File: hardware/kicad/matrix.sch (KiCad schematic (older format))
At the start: 14 parts

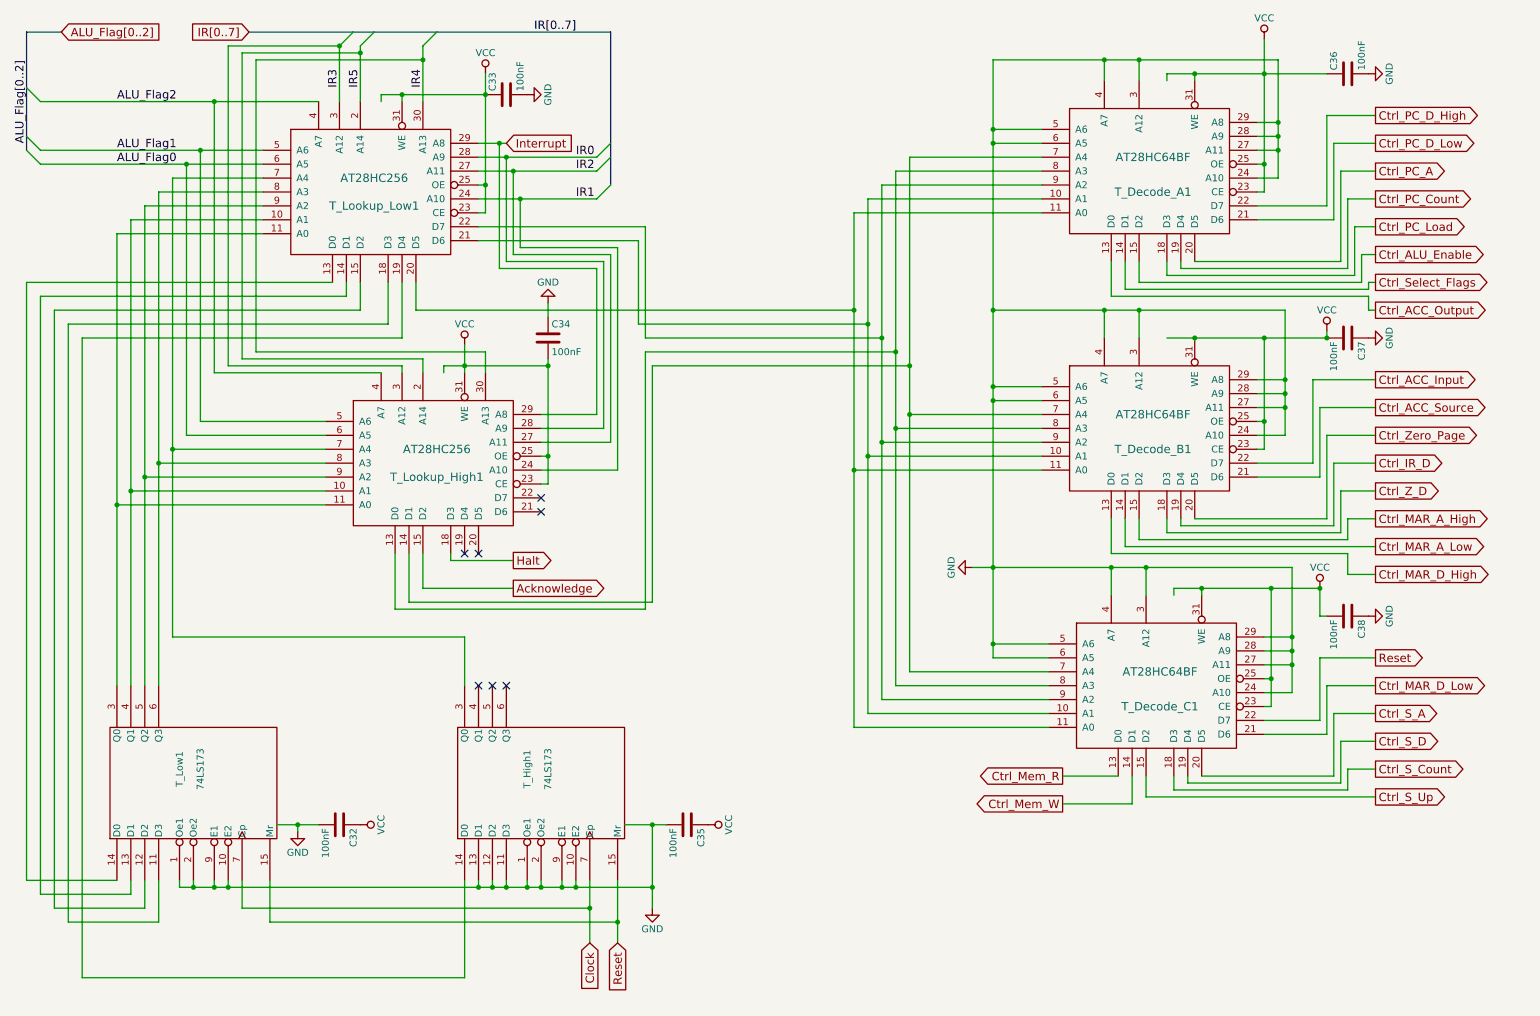
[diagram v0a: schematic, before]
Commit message: Just a backup.
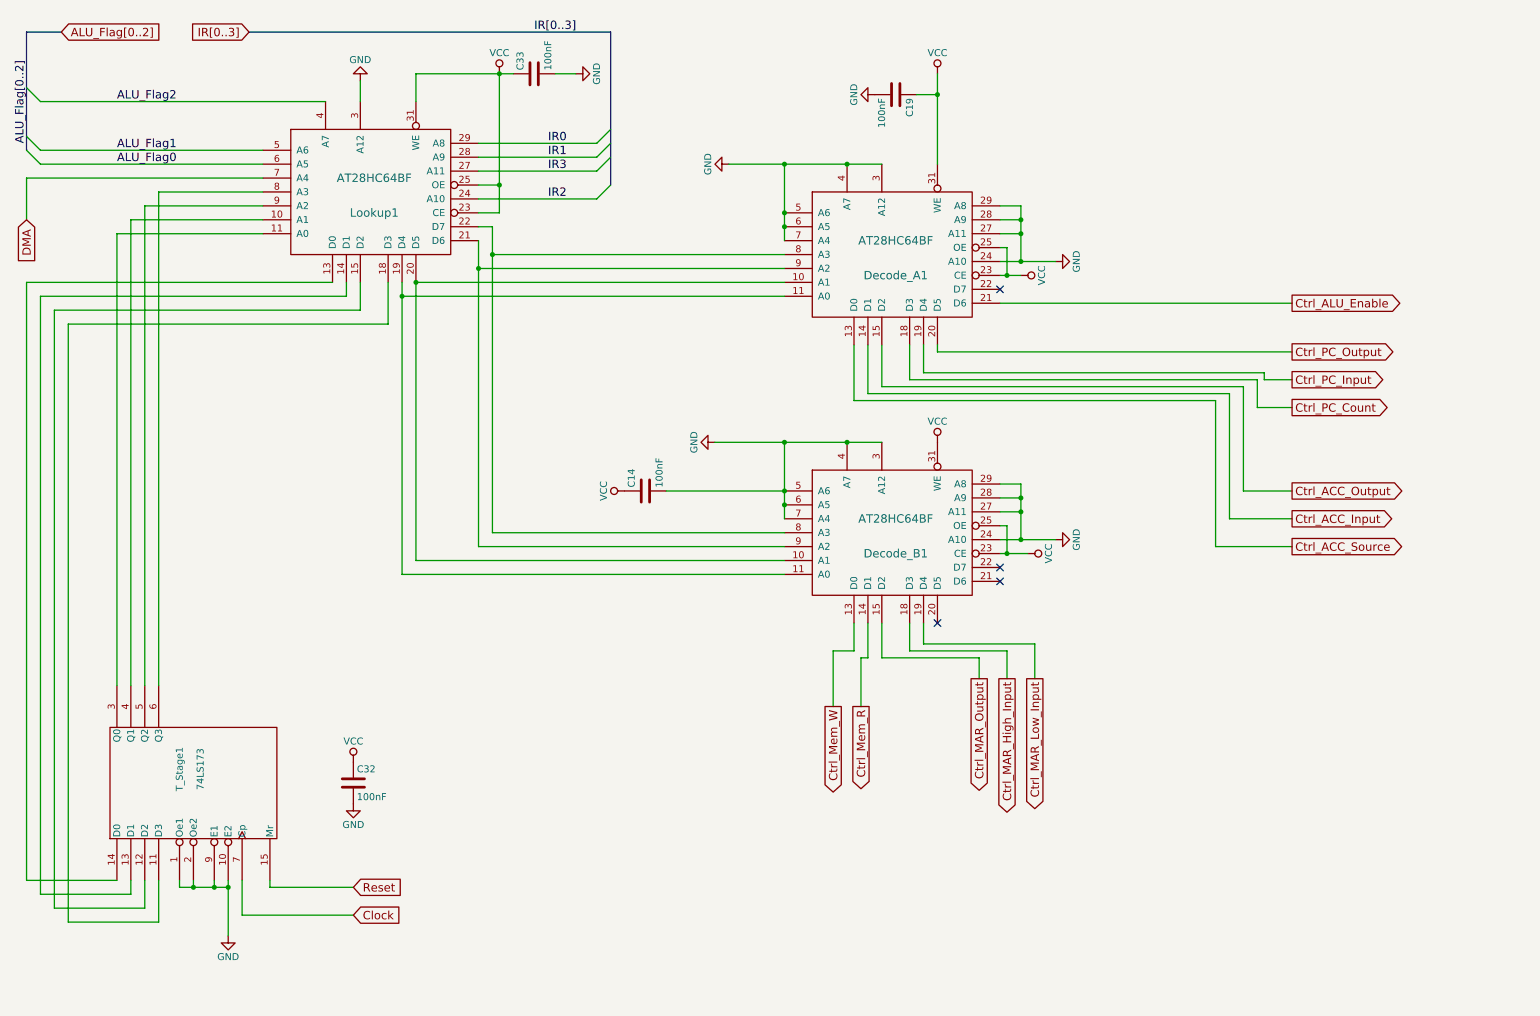
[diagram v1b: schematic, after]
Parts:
- removed C34, C35, C36, C37, C38: 100nF, Capacitors_THT:C_Disc_D5.0mm_W2.5mm_P2.50mm, symbol C
- removed T_Decode_A1, T_Decode_B1, T_Decode_C1: AT28HC64BF, PLCC32_bugfix:PLCC-32_THT-Socket_bugfix, symbol AT28HC64BF
- removed T_High1: 74LS173, Housings_DIP:DIP-16_W7.62mm, symbol 74LS173
- removed T_Lookup_High1, T_Lookup_Low1: AT28HC256, PLCC32_bugfix:PLCC-32_THT-Socket_bugfix, symbol AT28HC256
- added C14, C19: 100nF, Capacitors_ThroughHole:C_Disc_D3_P2.5, symbol C
- added Decode_A1, Decode_B1, Lookup1: AT28HC64BF, PLCC32_bugfix:PLCC-32_THT-Socket_bugfix, symbol AT28HC64BF
- C32, C33: footprint Capacitors_THT:C_Disc_D5.0mm_W2.5mm_P2.50mm -> Capacitors_ThroughHole:C_Disc_D3_P2.5
- renumbered T_Low1 to T_Stage1
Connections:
- net ALU_Flag0: now also Lookup1.6 (A5)
- net ALU_Flag1: now also Lookup1.5 (A6)
- net ALU_Flag2: now also Lookup1.4 (A7)
- net Ctrl_ACC_Input: now also Decode_A1.14 (D1)
- net Ctrl_ACC_Output: now also Decode_A1.15 (D2)
- net Ctrl_ACC_Source: now also Decode_A1.13 (D0)
- net Ctrl_ALU_Enable: now also Decode_A1.21 (D6)
- net Ctrl_Mem_R: now also Decode_B1.14 (D1)
- net Ctrl_Mem_W: now also Decode_B1.13 (D0)
- net Ctrl_PC_Count: now also Decode_A1.18 (D3)
- net GND: now also C14.2, C19.2, Decode_A1.16 (GND), Decode_A1.24 (A10), Decode_A1.27 (A11), Decode_A1.28 (A9), Decode_A1.29 (A8), Decode_A1.3 (A12), Decode_A1.4 (A7), Decode_A1.5 (A6), Decode_A1.6 (A5), Decode_A1.7 (A4), Decode_B1.16 (GND), Decode_B1.24 (A10), Decode_B1.27 (A11), Decode_B1.28 (A9), Decode_B1.29 (A8), Decode_B1.3 (A12), Decode_B1.4 (A7), Decode_B1.5 (A6), Decode_B1.6 (A5), Decode_B1.7 (A4), Lookup1.16 (GND), Lookup1.3 (A12)
- net IR0: now also Lookup1.29 (A8)
- net IR1: now also Lookup1.28 (A9)
- net IR2: now also Lookup1.24 (A10)
- net IR3: now also Lookup1.27 (A11)
- net VCC: now also C14.1, C19.1, Decode_A1.23 (CE), Decode_A1.25 (OE), Decode_A1.31 (WE), Decode_A1.32 (VCC), Decode_B1.23 (CE), Decode_B1.25 (OE), Decode_B1.31 (WE), Decode_B1.32 (VCC), Lookup1.23 (CE), Lookup1.25 (OE), Lookup1.31 (WE), Lookup1.32 (VCC)
- net at T_Stage1.4 (Q1): now also Lookup1.10 (A1)
- net at T_Stage1.3 (Q0): now also Lookup1.11 (A0)
- net at T_Stage1.14 (D0): now also Lookup1.13 (D0)
- net at T_Stage1.13 (D1): now also Lookup1.14 (D1)
- net at T_Stage1.12 (D2): now also Lookup1.15 (D2)
- net at T_Stage1.11 (D3): now also Lookup1.18 (D3)
- net at T_Stage1.6 (Q3): now also Lookup1.8 (A3)
- net at T_Stage1.5 (Q2): now also Lookup1.9 (A2)
- new net: Decode_A1.11 (A0), Decode_B1.11 (A0), Lookup1.19 (D4)
- new net: Decode_A1.10 (A1), Decode_B1.10 (A1), Lookup1.20 (D5)
- new net: Decode_A1.9 (A2), Decode_B1.9 (A2), Lookup1.21 (D6)
- new net: Decode_A1.8 (A3), Decode_B1.8 (A3), Lookup1.22 (D7)
- new net Ctrl_MAR_High_Input: Decode_B1.18 (D3)
- new net Ctrl_MAR_Low_Input: Decode_B1.19 (D4)
- new net Ctrl_MAR_Output: Decode_B1.15 (D2)
- new net Ctrl_PC_Input: Decode_A1.19 (D4)
- new net Ctrl_PC_Output: Decode_A1.20 (D5)
- new net DMA: Lookup1.7 (A4)
- no-connect marks 7 -> 4
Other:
- moved on the sheet: C32, C33

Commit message: Just a backup.
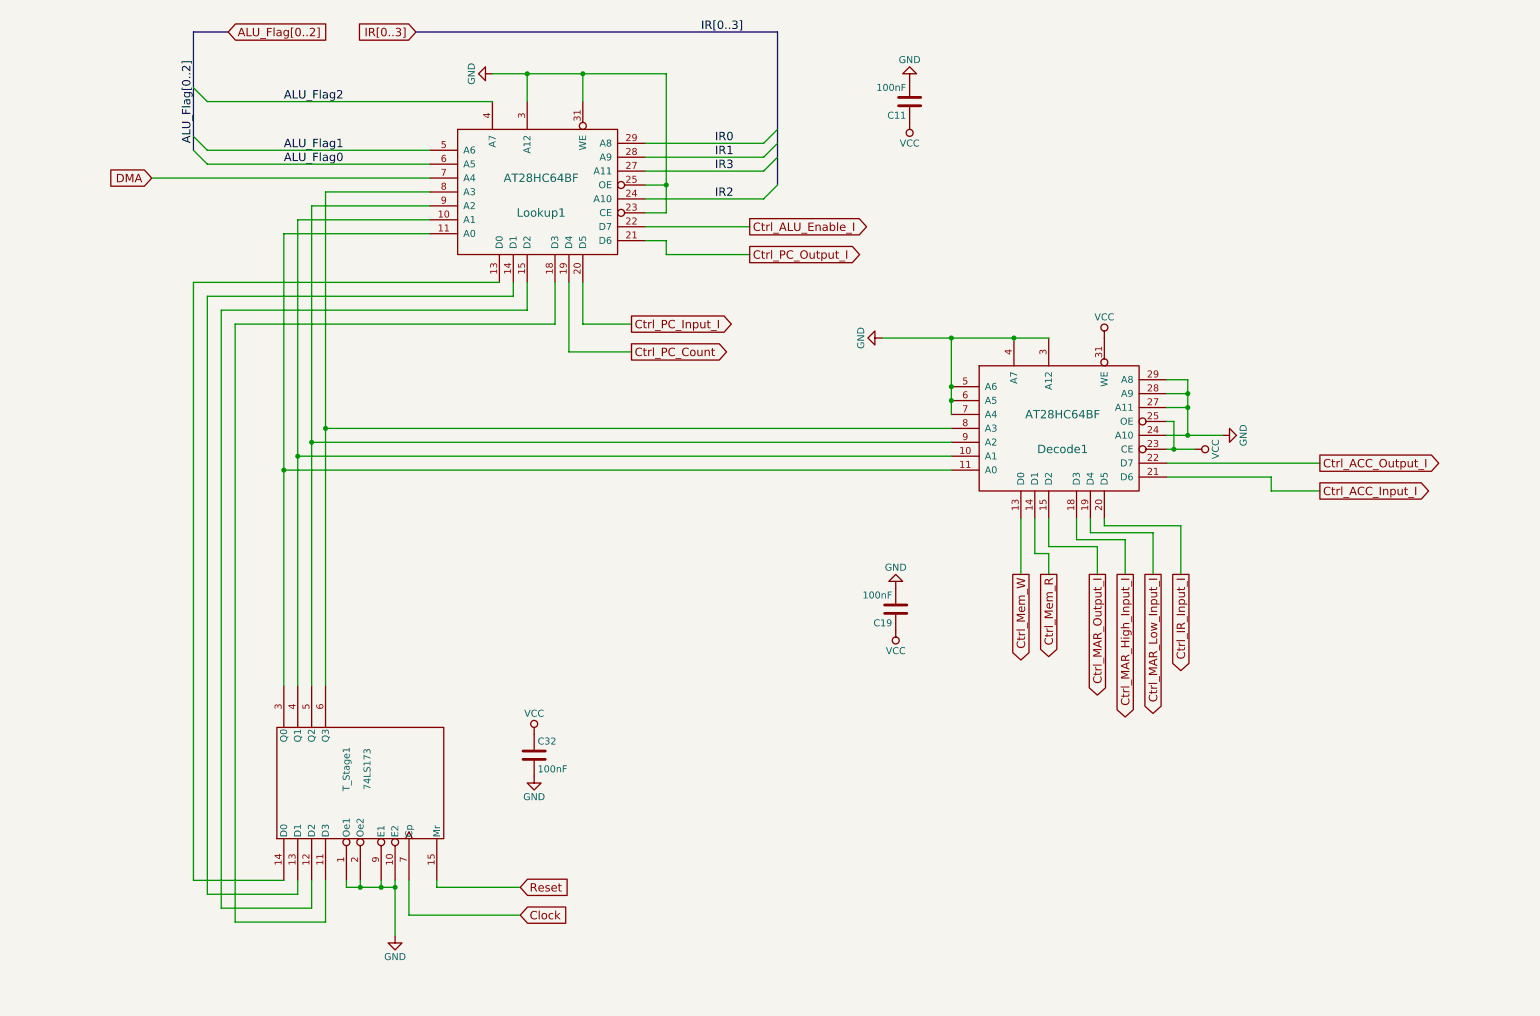
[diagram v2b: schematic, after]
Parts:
- removed C14, C33: 100nF, Capacitors_ThroughHole:C_Disc_D3_P2.5, symbol C
- removed Decode_A1: AT28HC64BF, PLCC32_bugfix:PLCC-32_THT-Socket_bugfix, symbol AT28HC64BF
- added C11: 100nF, Capacitors_ThroughHole:C_Disc_D3_P2.5, symbol C
- renumbered Decode_B1 to Decode1
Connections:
- net Ctrl_PC_Count: now also Lookup1.19 (D4)
- net GND: now also Lookup1.23 (CE), Lookup1.25 (OE), Lookup1.31 (WE), C11.2
- net VCC: now also C11.1; no longer Lookup1.23 (CE), Lookup1.25 (OE), Lookup1.31 (WE)
- net at Lookup1.11 (A0), T_Stage1.3 (Q0): now also Decode1.11 (A0)
- net at Lookup1.10 (A1), T_Stage1.4 (Q1): now also Decode1.10 (A1)
- net at Lookup1.9 (A2), T_Stage1.5 (Q2): now also Decode1.9 (A2)
- net at Lookup1.8 (A3), T_Stage1.6 (Q3): now also Decode1.8 (A3)
- net Ctrl_PC_Input_I: now reaches Lookup1.20 (D5)
- net Ctrl_PC_Input_I: no longer Decode1.10 (A1)
- net Ctrl_PC_Output_I: now reaches Lookup1.21 (D6)
- net Ctrl_PC_Output_I: no longer Decode1.9 (A2)
- net Ctrl_ALU_Enable_I: now reaches Lookup1.22 (D7)
- net Ctrl_ALU_Enable_I: no longer Decode1.8 (A3)
- net Ctrl_IR_Input_I: now reaches Decode1.20 (D5)
- net Ctrl_ACC_Input_I: now reaches Decode1.21 (D6)
- net Ctrl_ACC_Output_I: now reaches Decode1.22 (D7)
- net Ctrl_MAR_High_Input renamed Ctrl_MAR_High_Input_I
- net Ctrl_MAR_Low_Input renamed Ctrl_MAR_Low_Input_I
- net Ctrl_MAR_Output renamed Ctrl_MAR_Output_I
- no-connect marks 4 -> 0
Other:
- moved on the sheet: C32, Decode1, Lookup1, T_Stage1
